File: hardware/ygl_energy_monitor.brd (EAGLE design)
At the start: 50.8 x 52 mm, 5 parts

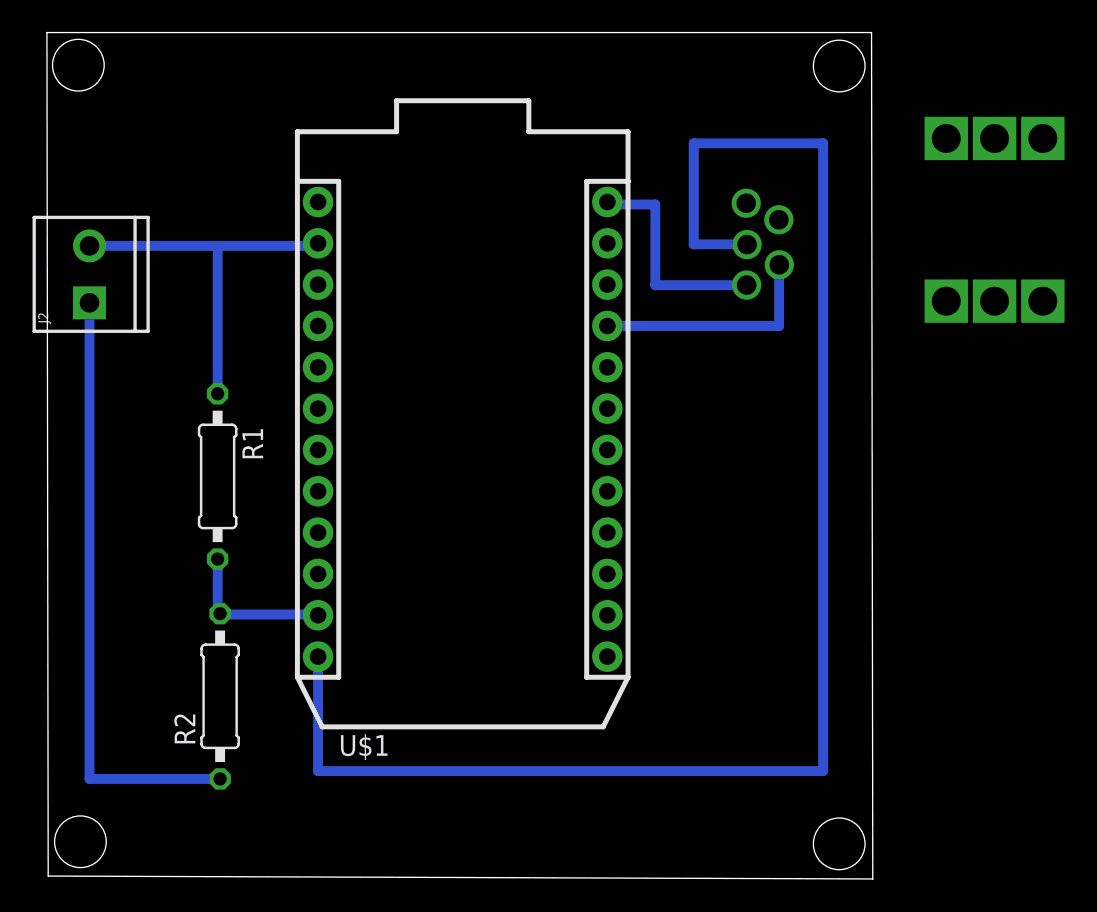
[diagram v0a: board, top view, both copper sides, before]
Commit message: fixed package
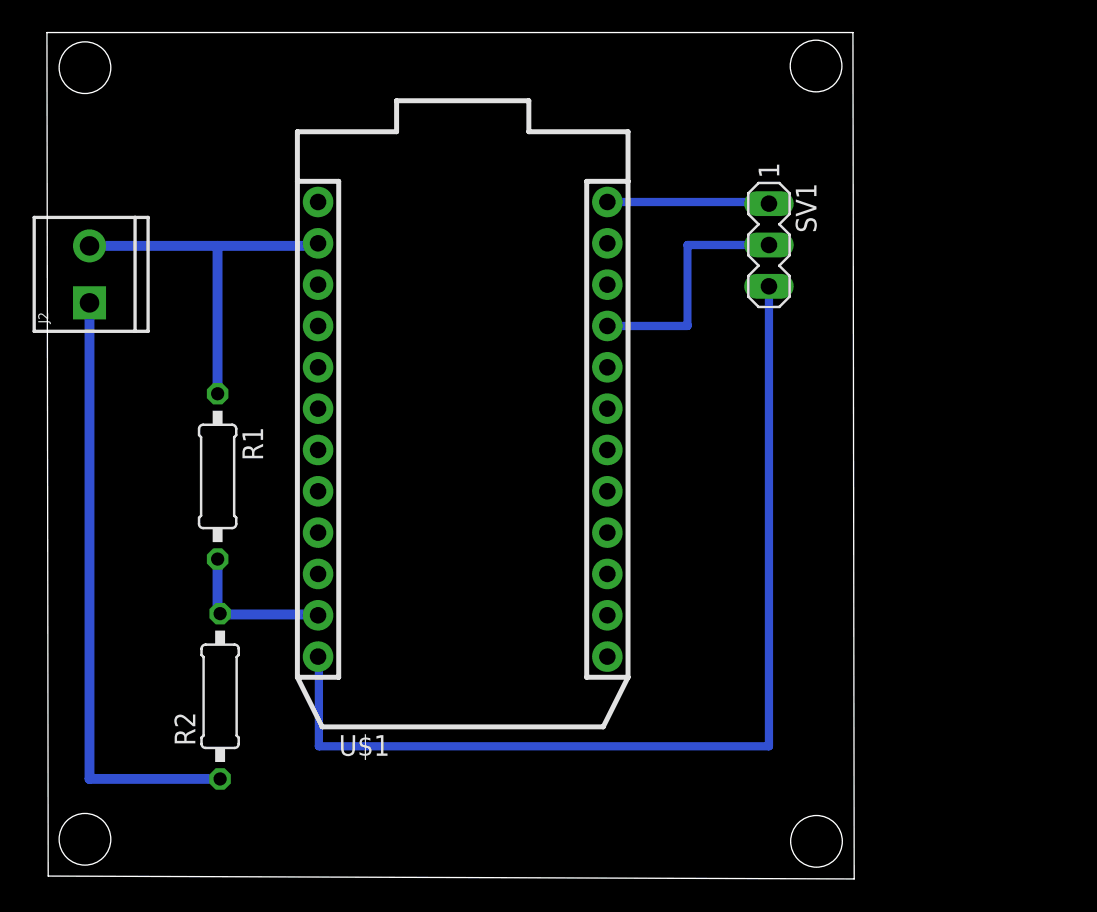
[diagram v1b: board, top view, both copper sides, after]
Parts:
- removed U$2: (no value), LEM:HO6SP33
- added SV1: (no value), con-lstb:MA03-1
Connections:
- net N$1: now also SV1.1; no longer U$2.V_CC
- net N$2: now also SV1.2; no longer U$2.GND
- net N$3: now also SV1.3; no longer U$2.V_OUT
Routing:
- net N$3: track 94.1 -> 61.5 mm
- net N$1: track 13.7 -> 10.2 mm
- net N$2: track 14.9 -> 15.5 mm
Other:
- board size 50.8 x 52 mm -> 49.6 x 52 mm
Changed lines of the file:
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@@
 <board>
 <plain>
-<wire x1="-0.0762" y1="8.6106" x2="50.6022" y2="8.4328" width="0" layer="20"/>
-<wire x1="50.6022" y1="8.4328" x2="50.526" y2="60.4522" width="0" layer="20"/>
-<wire x1="50.526" y1="60.4522" x2="-0.1524" y2="60.4522" width="0" layer="20"/>
+<wire x1="-0.0762" y1="8.6106" x2="49.4592" y2="8.4328" width="0" layer="20"/>
+<wire x1="49.4592" y1="8.4328" x2="49.383" y2="60.4522" width="0" layer="20"/>
+<wire x1="49.383" y1="60.4522" x2="-0.1524" y2="60.4522" width="0" layer="20"/>
 <wire x1="-0.1524" y1="60.4522" x2="-0.0762" y2="8.6106" width="0" layer="20"/>
-<hole x="1.778" y="58.4454" drill="3.175"/>
-<hole x="1.905" y="10.7188" drill="3.175"/>
-<hole x="48.5394" y="10.5918" drill="3.175"/>
-<hole x="48.5394" y="58.3946" drill="3.175"/>
+<hole x="2.1844" y="58.293" drill="3.175"/>
+<hole x="2.1844" y="10.8712" drill="3.175"/>
+<hole x="47.1424" y="10.7442" drill="3.175"/>
+<hole x="47.117" y="58.3946" drill="3.175"/>
 </plain>
 <attributes>
@@
 </autorouter>
 <elements>
-<element name="U$2" library="LEM" package="HO6SP33" value="" x="55.118" y="43.942" rot="R270"/>
 <element name="U$1" library="Spark" package="PHOTON" value="PHOTON_WITH_HEADERS" x="15.24" y="17.78"/>
 <element name="J2" library="SparkFun-Connectors" package="SCREWTERMINAL-3.5MM-2" value="" x="2.4638" y="43.8404" rot="R90">
@@
 <element name="R2" library="resistor" library_urn="urn:adsk.eagle:library:348" package="0207/10" package3d_urn="urn:adsk.eagle:package:25939/1" value="" x="10.4902" y="19.6596" rot="R90"/>
 <element name="R1" library="resistor" library_urn="urn:adsk.eagle:library:348" package="0207/10" package3d_urn="urn:adsk.eagle:package:25939/1" value="" x="10.3378" y="33.1724" rot="R270"/>
+<element name="SV1" library="con-lstb" library_urn="urn:adsk.eagle:library:162" package="MA03-1" package3d_urn="urn:adsk.eagle:package:8339/1" value="" x="44.2214" y="47.3964" rot="R270">
+<attribute name="MF" value="" x="44.2214" y="47.3964" size="1.778" layer="27" rot="R270" display="off"/>
+<attribute name="MPN" value="" x="44.2214" y="47.3964" size="1.778" layer="27" rot="R270" display="off"/>
+<attribute name="OC_FARNELL" value="unknown" x="44.2214" y="47.3964" size="1.778" layer="27" rot="R270" display="off"/>
+<attribute name="OC_NEWARK" value="unknown" x="44.2214" y="47.3964" size="1.778" layer="27" rot="R270" display="off"/>
+</element>
 </elements>
 <signals>
@@
 <signal name="N$1">
 <contactref element="U$1" pad="24"/>
-<contactref element="U$2" pad="V_CC"/>
-<wire x1="42.848" y1="44.926" x2="37.2364" y2="44.926" width="0.6096" layer="16"/>
-<wire x1="37.2364" y1="44.926" x2="37.2364" y2="49.8856" width="0.6096" layer="16"/>
-<wire x1="37.2364" y1="49.8856" x2="34.29" y2="49.8856" width="0.6096" layer="16"/>
 <wire x1="34.29" y1="49.8856" x2="34.29" y2="50.038" width="0.6096" layer="16"/>
+<contactref element="SV1" pad="1"/>
+<wire x1="34.29" y1="50.038" x2="44.2214" y2="50.038" width="0.508" layer="16"/>
+<wire x1="44.2214" y1="50.038" x2="44.2214" y2="49.9364" width="0.508" layer="16"/>
 </signal>
 <signal name="N$2">
 <contactref element="U$1" pad="21"/>
-<contactref element="U$2" pad="GND"/>
 <wire x1="34.4678" y1="42.5196" x2="34.544" y2="41.91" width="0.4064" layer="16"/>
-<wire x1="44.848" y1="46.18" x2="44.848" y2="42.418" width="0.6096" layer="16"/>
-<wire x1="44.848" y1="42.418" x2="34.29" y2="42.418" width="0.6096" layer="16"/>
+<contactref element="SV1" pad="2"/>
+<wire x1="34.29" y1="42.418" x2="39.2176" y2="42.418" width="0.508" layer="16"/>
+<wire x1="39.2176" y1="47.3964" x2="44.2214" y2="47.3964" width="0.508" layer="16"/>
+<wire x1="39.2176" y1="42.418" x2="39.2176" y2="47.3964" width="0.508" layer="16"/>
 <wire x1="34.29" y1="42.418" x2="34.4678" y2="42.5196" width="0" layer="19" extent="16-16"/>
 </signal>
 <signal name="N$3">
-<contactref element="U$2" pad="V_OUT"/>
 <contactref element="U$1" pad="12"/>
-<wire x1="47.5488" y1="15.0622" x2="47.5488" y2="53.6448" width="0.6096" layer="16"/>
-<wire x1="47.5488" y1="53.6448" x2="39.5986" y2="53.6448" width="0.6096" layer="16"/>
-<wire x1="39.5986" y1="53.6448" x2="39.5986" y2="47.434" width="0.6096" layer="16"/>
-<wire x1="39.5986" y1="47.434" x2="42.848" y2="47.434" width="0.6096" layer="16"/>
-<wire x1="16.51" y1="22.098" x2="16.51" y2="15.0622" width="0.6096" layer="16"/>
-<wire x1="16.51" y1="15.0622" x2="47.5488" y2="15.0622" width="0.6096" layer="16"/>
-</signal>
-<signal name="N$8">
-<via x="42.8244" y="49.9618" extent="1-16" drill="1.2" diameter="0.8128"/>
-</signal>
-<signal name="N$9">
-<via x="44.831" y="48.9458" extent="1-16" drill="1.2" diameter="0.8128"/>
-</signal>
-<signal name="N$10">
-<via x="42.8752" y="47.4218" extent="1-16" drill="1.2" diameter="0.8128"/>
-</signal>
-<signal name="N$11">
-<via x="44.8564" y="46.1772" extent="1-16" drill="1.2" diameter="0.8128"/>
-</signal>
-<signal name="N$12">
-<via x="42.8498" y="44.9326" extent="1-16" drill="1.2" diameter="0.8128"/>
+<contactref element="SV1" pad="3"/>
+<wire x1="44.2214" y1="44.8564" x2="44.2214" y2="16.5862" width="0.508" layer="16"/>
+<wire x1="44.2214" y1="16.5862" x2="16.5608" y2="16.5862" width="0.508" layer="16"/>
+<wire x1="16.5608" y1="16.5862" x2="16.5608" y2="22.098" width="0.508" layer="16"/>
+<wire x1="16.5608" y1="22.098" x2="16.51" y2="22.098" width="0.508" layer="16"/>
 </signal>
 <signal name="VIN">
